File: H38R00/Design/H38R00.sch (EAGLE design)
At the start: 38 parts, among them P1 HEXABIT_17.32_X2_POWER_ONLY, U1 LM5160DNT, U2 TPS65130RGERT, X1 INPUT, X2 OUT-15P, X3 OUT-15N, X4 OUT-5P

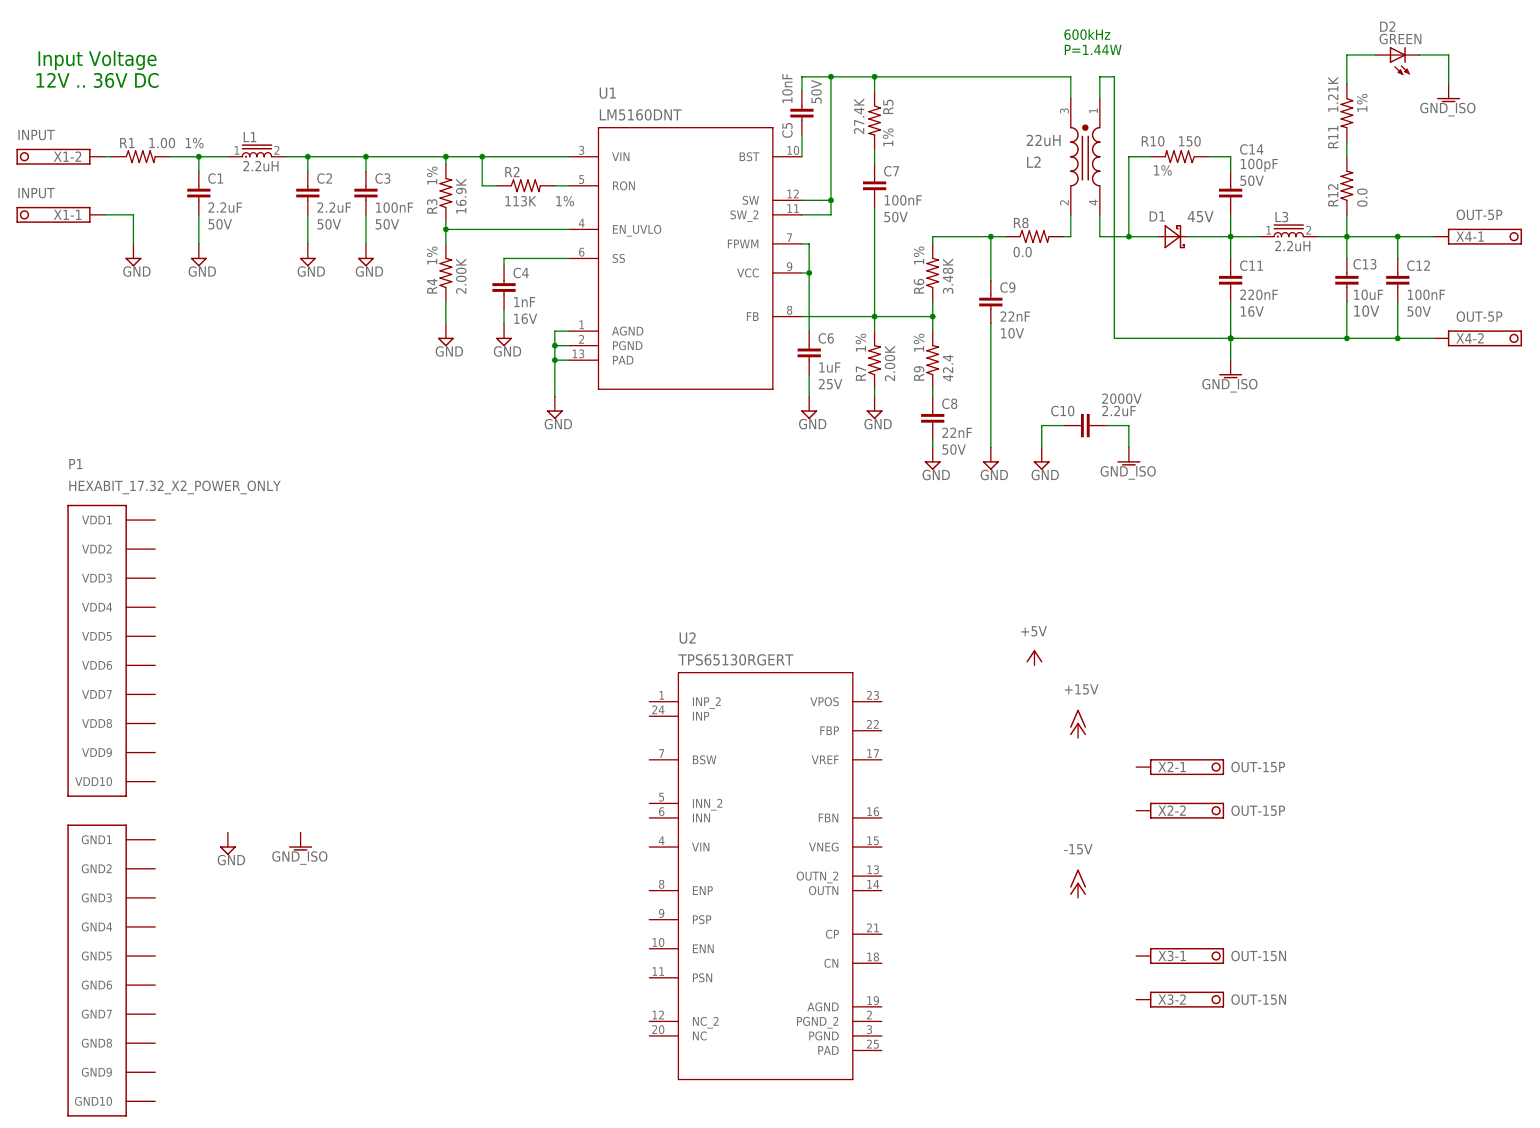
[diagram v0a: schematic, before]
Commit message: Finished schematics
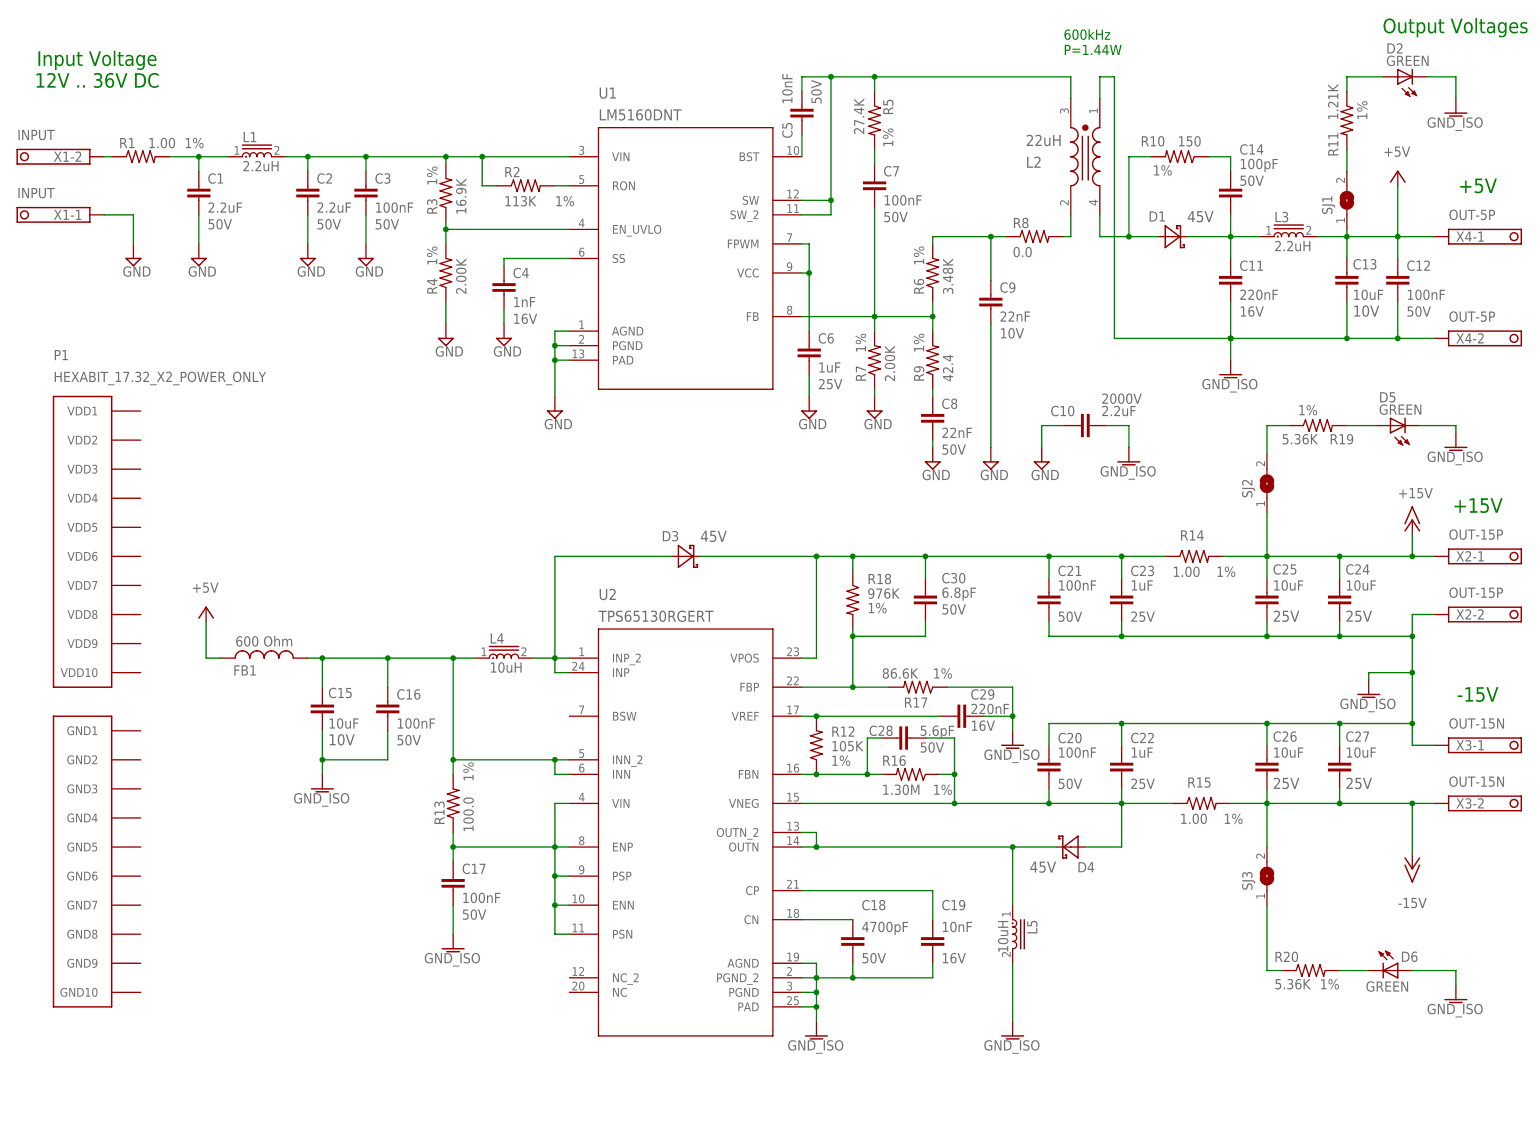
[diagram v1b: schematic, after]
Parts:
- added C15, C24, C25, C26, C27: 10uF, Hexabitz:C-0805
- added C16, C17, C20, C21: 100nF, Hexabitz:C-0603
- added C18: 4700pF, Hexabitz:C-0603
- added C19: 10nF, Hexabitz:C-0603
- added C22, C23: 1uF, Hexabitz:C-0603
- added C28: 5.6pF, Hexabitz:C-0603
- added C29: 220nF, Hexabitz:C-0603
- added C30: 6.8pF, Hexabitz:C-0603
- added D3, D4: DIOD-SOD-123, Hexabitz:DIOD-SOD-123
- added D5, D6: GREEN, Hexabitz:VLMTG1300-GS08
- added FB1: 600 Ohm, Hexabitz:FB-0603
- added L4, L5: 10uH, Hexabitz:WUERTH_ELEKTRONIK_74404024100WUERTH_ELEKTRONIK_74404024100_0_0
- added R13: 100.0, Hexabitz:R-0603
- added R14, R15: 1.00, Hexabitz:R-0603
- added R16: 1.30M, Hexabitz:R-0603
- added R17: 86.6K, Hexabitz:R-0603
- added R18: 976K, Hexabitz:R-0603
- added R19, R20: 5.36K, Hexabitz:R-0603
- added SJ1, SJ2, SJ3: (no value), jumper:SJ
- R12: value 0.0 -> 105K; MFN Panasonic -> Vishay; MPN ERJ-3GEY0R00V -> CRCW0603105KFKEA; OCTOPART_URL https://octopart.com/erj-3gey0r00v-panasonic-55389238?r=sp&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 -> https://octopart.com/crcw0603105kfkea-vishay-39783419?r=sp&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; RESISTANCE 0.0R -> 105K; TOLERANCE 5% -> 1%
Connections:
- new net +15V: C24.1, C25.1, R14.2, SJ2.1, X2-1.K
- new net +5V: C12.1, C13.1, FB1.1, L3.2, SJ1.1, X4-1.K
- new net -15V: C26.2, C27.2, R15.2, SJ3.2, X3-2.K
- new net N$21: D3.A, L4.2, U2.INP, U2.INP_2
- new net N$22: C21.1, C23.1, C30.2, D3.C, R14.1, R18.1, U2.VPOS
- new net N$23: C17.1, R13.1, U2.ENN, U2.ENP, U2.PSN, U2.PSP, U2.VIN
- new net N$24: C18.1, U2.CN
- new net N$25: C19.1, U2.CP
- new net N$26: D4.C, L5.1, U2.OUTN, U2.OUTN_2
- new net N$27: C20.2, C22.2, C28.2, D4.A, R15.1, R16.1, U2.VNEG
- new net N$28: C28.1, R12.1, R16.2, U2.FBN
- new net N$29: C29.1, R12.2, U2.VREF
- new net N$30: C30.1, R17.2, R18.2, U2.FBP
- new net N$31: R19.1, SJ2.2
- new net N$32: D5.A, R19.2
- new net N$33: R20.1, SJ3.1
- new net N$34: D6.C, R20.2
- net AGND: now also C15.2, C16.2, C17.2, C18.2, C19.2, C20.1, C21.2, C22.1, C23.2, C24.2, C25.2, C26.1, C27.1, C29.2, D5.C, D6.A, L5.2, R17.1, U2.AGND, U2.PAD, U2.PGND, U2.PGND_2, X2-2.K, X3-1.K
- net N$18: now also C15.1, C16.1, FB1.2, L4.1, R13.2, U2.INN, U2.INN_2; no longer C12.1, C13.1, L3.2, R12.1, X4-1.K
- net N$19: now also SJ1.2; no longer R12.2
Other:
- note added: "+15V"
- note added: "+5V"
- note added: "-15V"
- note added: "Output Voltages"
- moved on the sheet: D2, P1, R11, R12, U2, X2-1, X2-2, X3-1, X3-2
